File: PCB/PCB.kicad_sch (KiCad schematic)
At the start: 17 parts, among them U1 Buck Converter, U2 Ultrasonic Sensor, U4 Custom_ESP32_S3_Board

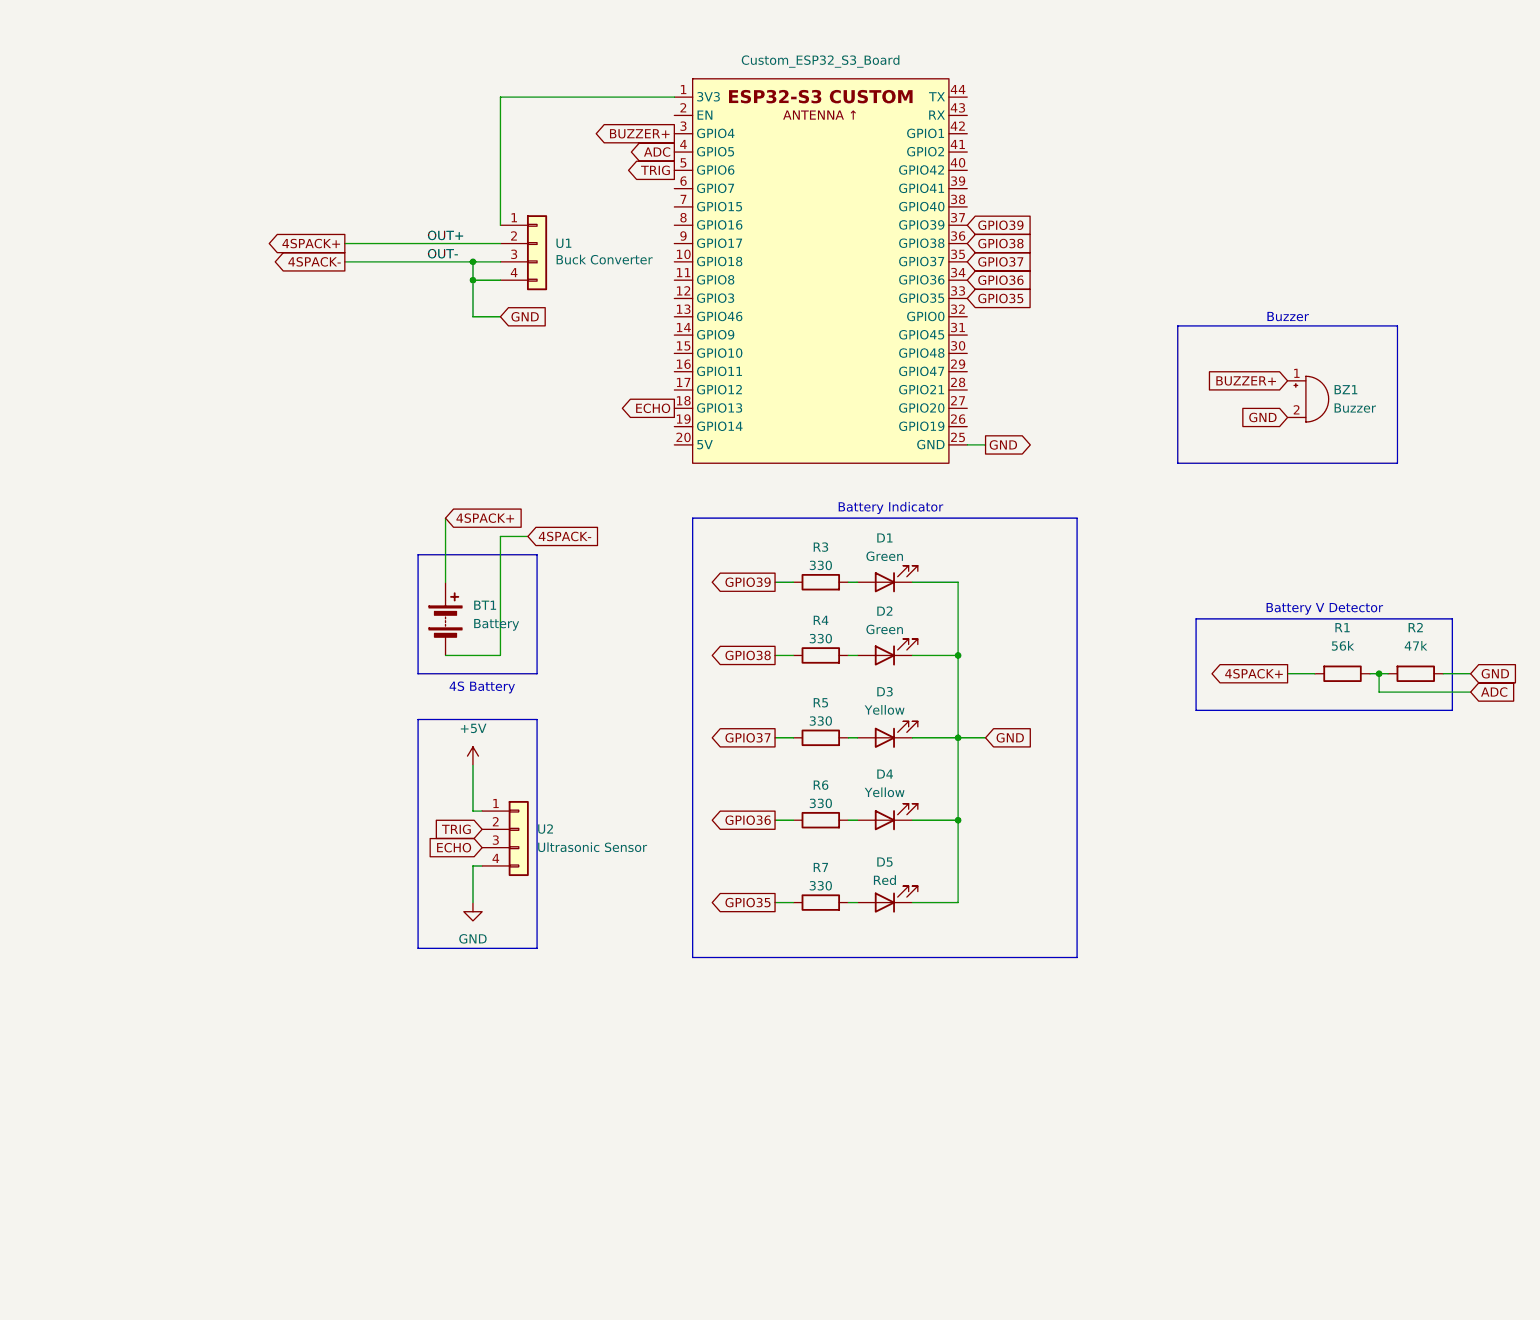
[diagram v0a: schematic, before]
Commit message: pcb
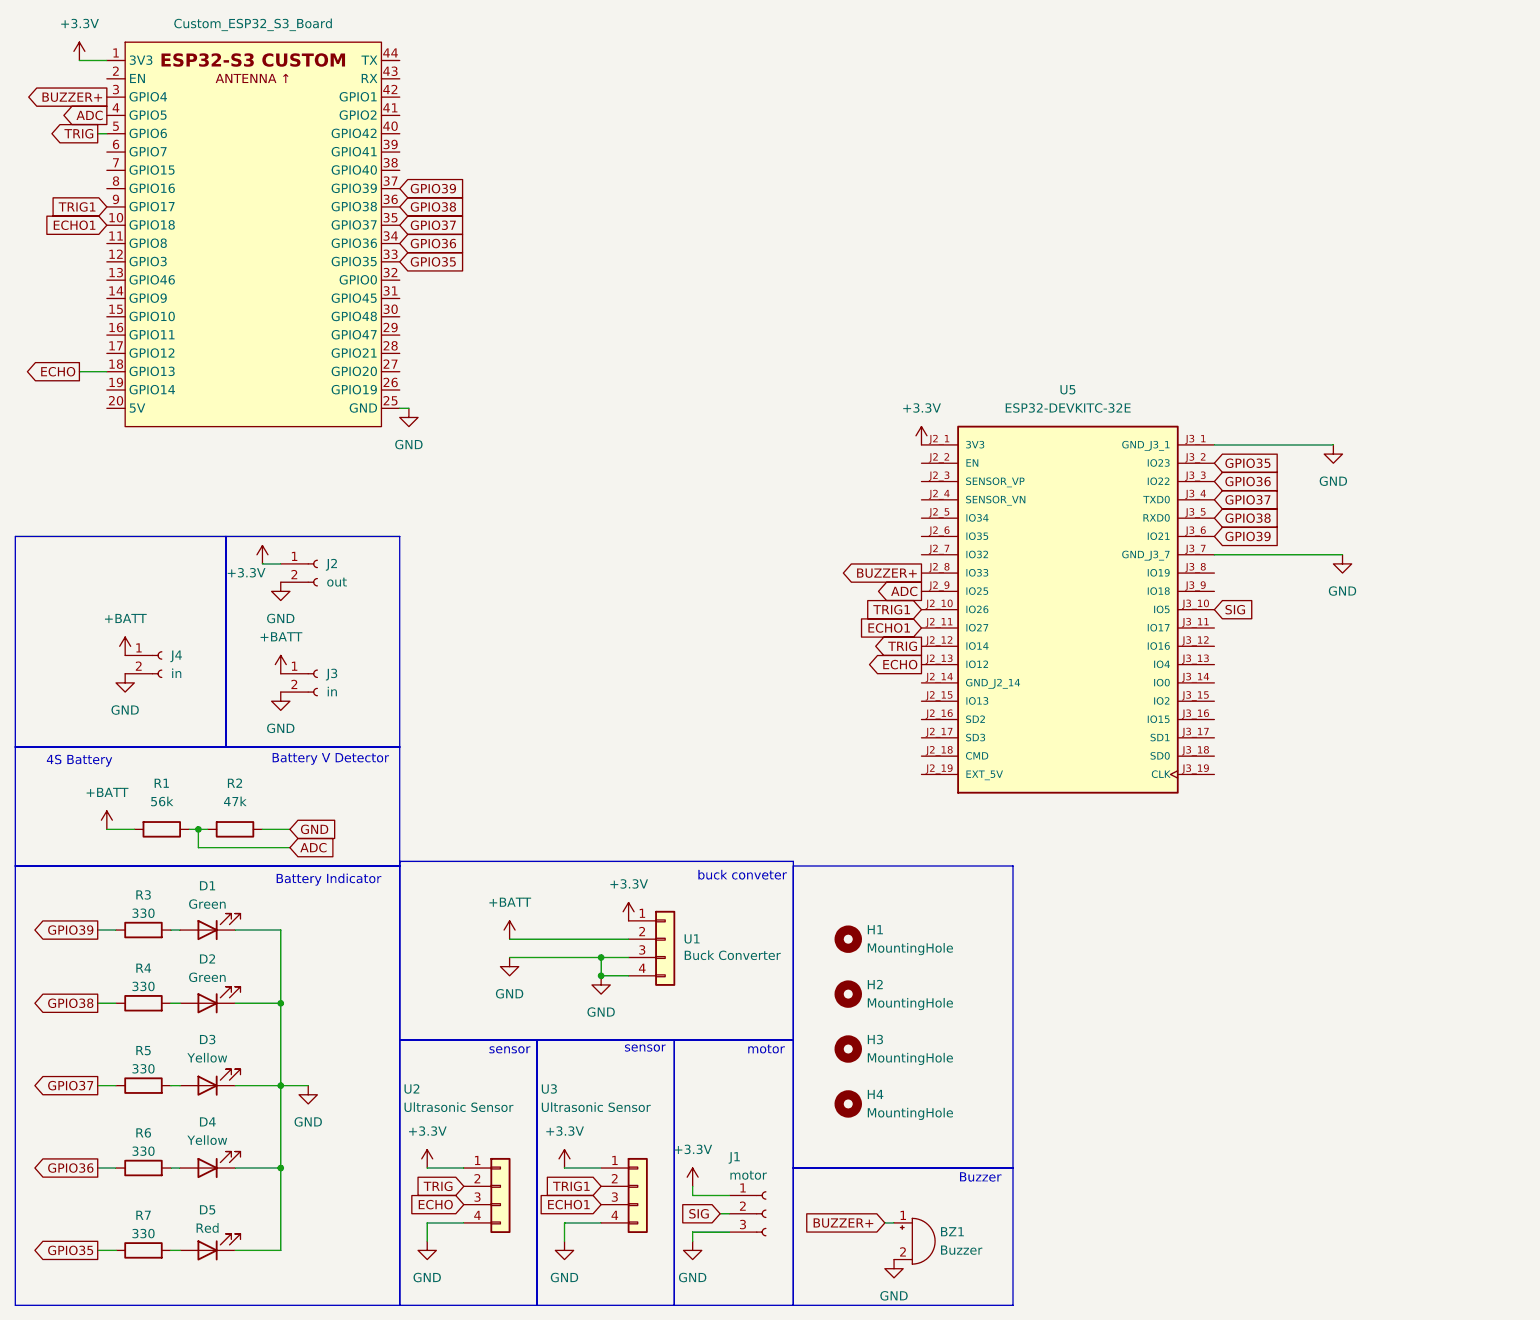
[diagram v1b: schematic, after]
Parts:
- removed BT1: Battery, Battery:BatteryHolder_Keystone_2462_2xAA, symbol Device:Battery
- added H1, H2, H3, H4: MountingHole, MountingHole:MountingHole_2.2mm_M2_DIN965, symbol Mechanical:MountingHole
- added J1: motor, Connector_PinHeader_2.54mm:PinHeader_1x03_P2.54mm_Vertical, symbol Connector:Conn_01x03_Socket
- added J2: out, Connector_PinHeader_2.54mm:PinHeader_1x02_P2.54mm_Vertical, symbol Connector:Conn_01x02_Socket
- added J3, J4: in, Connector_PinHeader_2.54mm:PinHeader_1x02_P2.54mm_Vertical, symbol Connector:Conn_01x02_Socket
- added U3: Ultrasonic Sensor, Connector_PinHeader_2.54mm:PinHeader_1x04_P2.54mm_Vertical, symbol Connector_Generic:Conn_01x04
- added U5: ESP32-DEVKITC-32E, ESP32-DEVKITC-32E:MODULE_ESP32-DEVKITC-32E, symbol ESP32-DEVKITC-32E:ESP32-DEVKITC-32E
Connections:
- net +5V is gone; now on net +3.3V: U2.1 (Pin_1)
- net ADC: now also U5.J2_9 (IO25)
- net BUZZER+: now also U5.J2_8 (IO33)
- net ECHO: now also U5.J2_13 (IO12)
- net GND: now also J1.3 (Pin_3), J2.2 (Pin_2), J3.2 (Pin_2), J4.2 (Pin_2), U3.4 (Pin_4), U5.J3_1 (GND_J3_1), U5.J3_7 (GND_J3_7)
- net GPIO35: now also U5.J3_2 (IO23)
- net GPIO36: now also U5.J3_3 (IO22)
- net GPIO37: now also U5.J3_4 (TXD0)
- net GPIO38: now also U5.J3_5 (RXD0)
- net GPIO39: now also U5.J3_6 (IO21)
- net TRIG: now also U5.J2_12 (IO14)
- net +3.3V: now reaches U1.1 (Pin_1), U4.1 (3V3)
- net +3.3V: now also J1.1 (Pin_1), J2.1 (Pin_1), U3.1 (Pin_1), U5.J2_1 (3V3)
- net ECHO1: now reaches U4.10 (GPIO18)
- net ECHO1: now also U3.3 (Pin_3), U5.J2_11 (IO27)
- net TRIG1: now reaches U4.9 (GPIO17)
- net TRIG1: now also U3.2 (Pin_2), U5.J2_10 (IO26)
- net 4SPACK+ renamed +BATT
- net +BATT: now also J3.1 (Pin_1), J4.1 (Pin_1)
- new net SIG: J1.2 (Pin_2), U5.J3_10 (IO5)
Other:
- note added: "buck conveter"
- note added: "motor"
- note added: "sensor"
- moved on the sheet: BZ1, D1, D2, D3, D4, D5, R1, R2, R3, R4, R5, R6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
